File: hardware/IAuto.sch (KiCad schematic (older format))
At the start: 4 parts, among them J6 Cable_PAD, J7 Cable_PAD, J8 Cable_PAD, J9 Cable_PAD

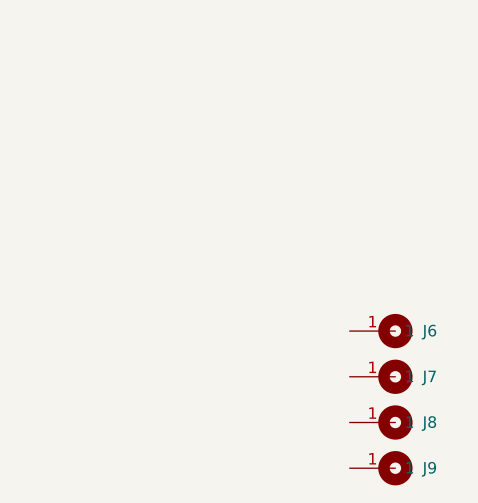
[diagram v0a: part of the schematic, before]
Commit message: ultimos cambios
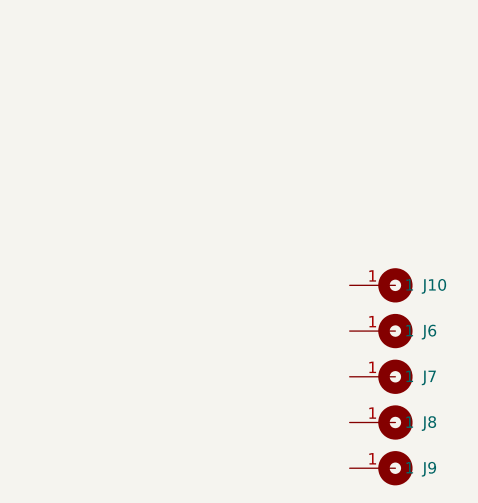
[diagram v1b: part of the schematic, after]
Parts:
- added J10: Cable_PAD, EESTN5:LOGO_EESTN5, symbol EESTN5:Cable_PAD
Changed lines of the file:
@@
+	1    0    0    -1
+$EndComp
+$Comp
+L EESTN5:Cable_PAD J10
+U 1 1 61432EC4
+P 10900 5600
+F 0 "J10" H 11019 5600 50  0000 L CNN
+F 1 "Cable_PAD" H 10900 5725 50  0001 C CNN
+F 2 "EESTN5:LOGO_EESTN5" H 10900 5600 60  0001 C CNN
+F 3 "" H 10900 5600 60  0001 C CNN
+	1    10900 5600
 	1    0    0    -1
 $EndComp

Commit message: Final
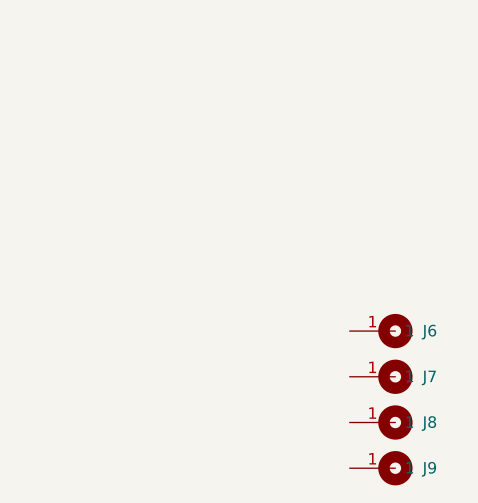
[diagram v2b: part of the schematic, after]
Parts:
- removed J10: Cable_PAD, EESTN5:LOGO_EESTN5, symbol EESTN5:Cable_PAD
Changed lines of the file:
@@
-	1    0    0    -1
-$EndComp
-$Comp
-L EESTN5:Cable_PAD J10
-U 1 1 61432EC4
-P 10900 5600
-F 0 "J10" H 11019 5600 50  0000 L CNN
-F 1 "Cable_PAD" H 10900 5725 50  0001 C CNN
-F 2 "EESTN5:LOGO_EESTN5" H 10900 5600 60  0001 C CNN
-F 3 "" H 10900 5600 60  0001 C CNN
-	1    10900 5600
 	1    0    0    -1
 $EndComp
